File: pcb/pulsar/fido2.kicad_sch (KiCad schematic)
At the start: 16 parts, among them J1 FPC_10P_0.5mm, U1 ISO1540DR, U2 STM32L052K8T6, U3 ATECC608B-MAHDA-S

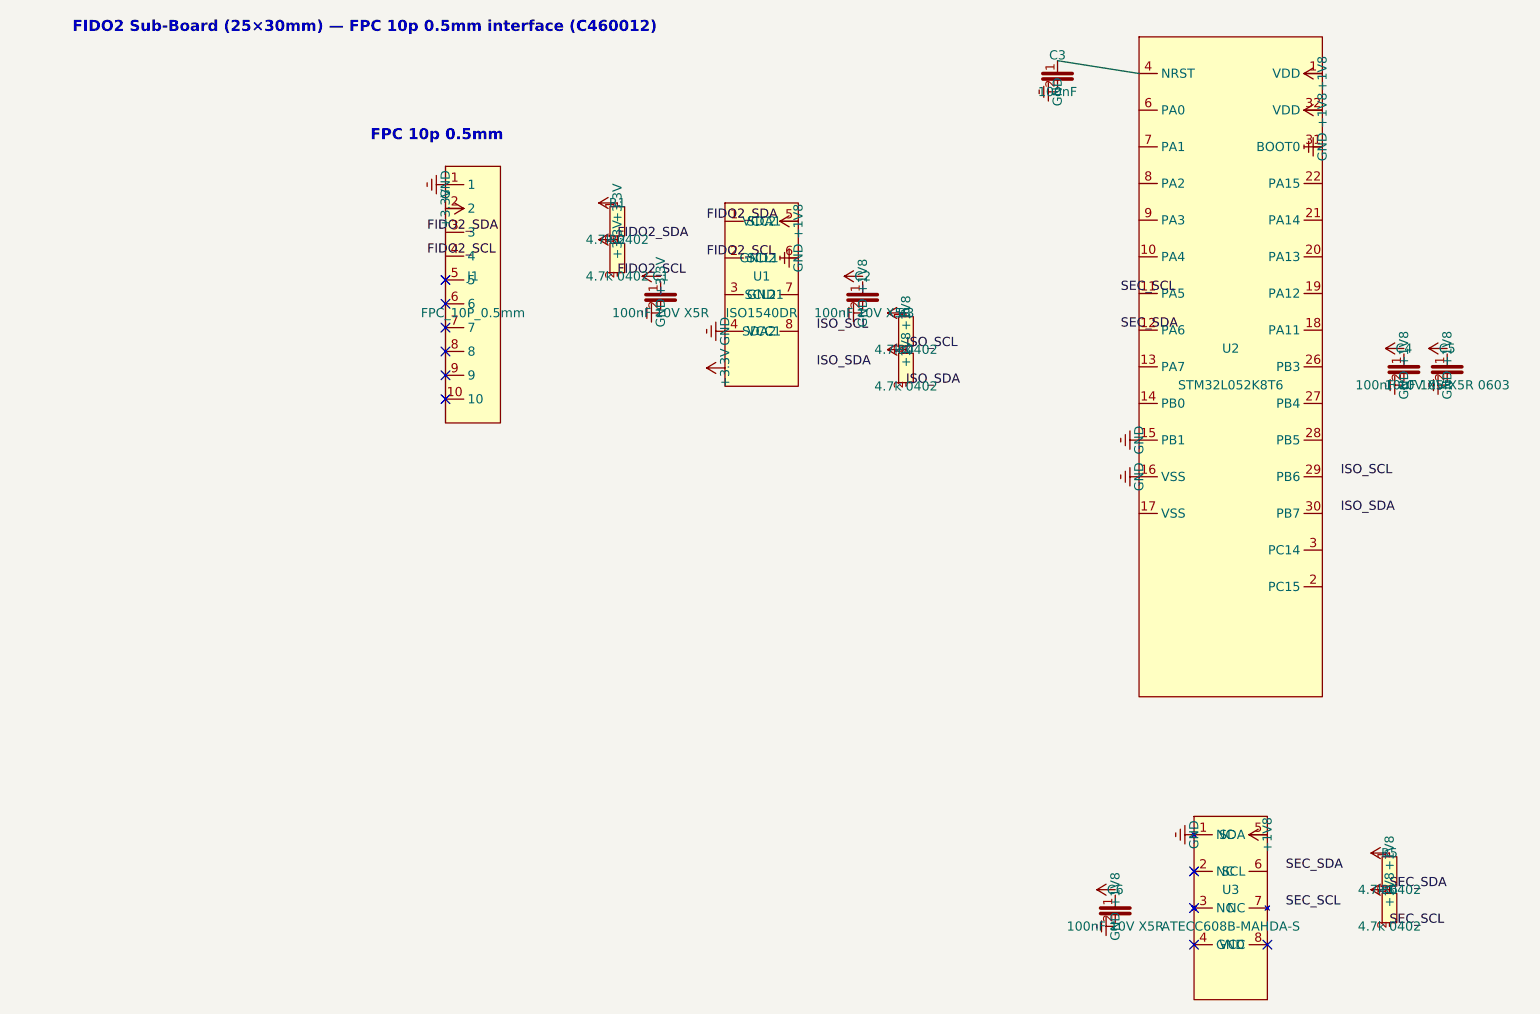
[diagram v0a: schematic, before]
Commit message: feat: let everything to route
Signed-off-by: Axel Ibarrondo <135344010+Axel84727@users.noreply.github.com>
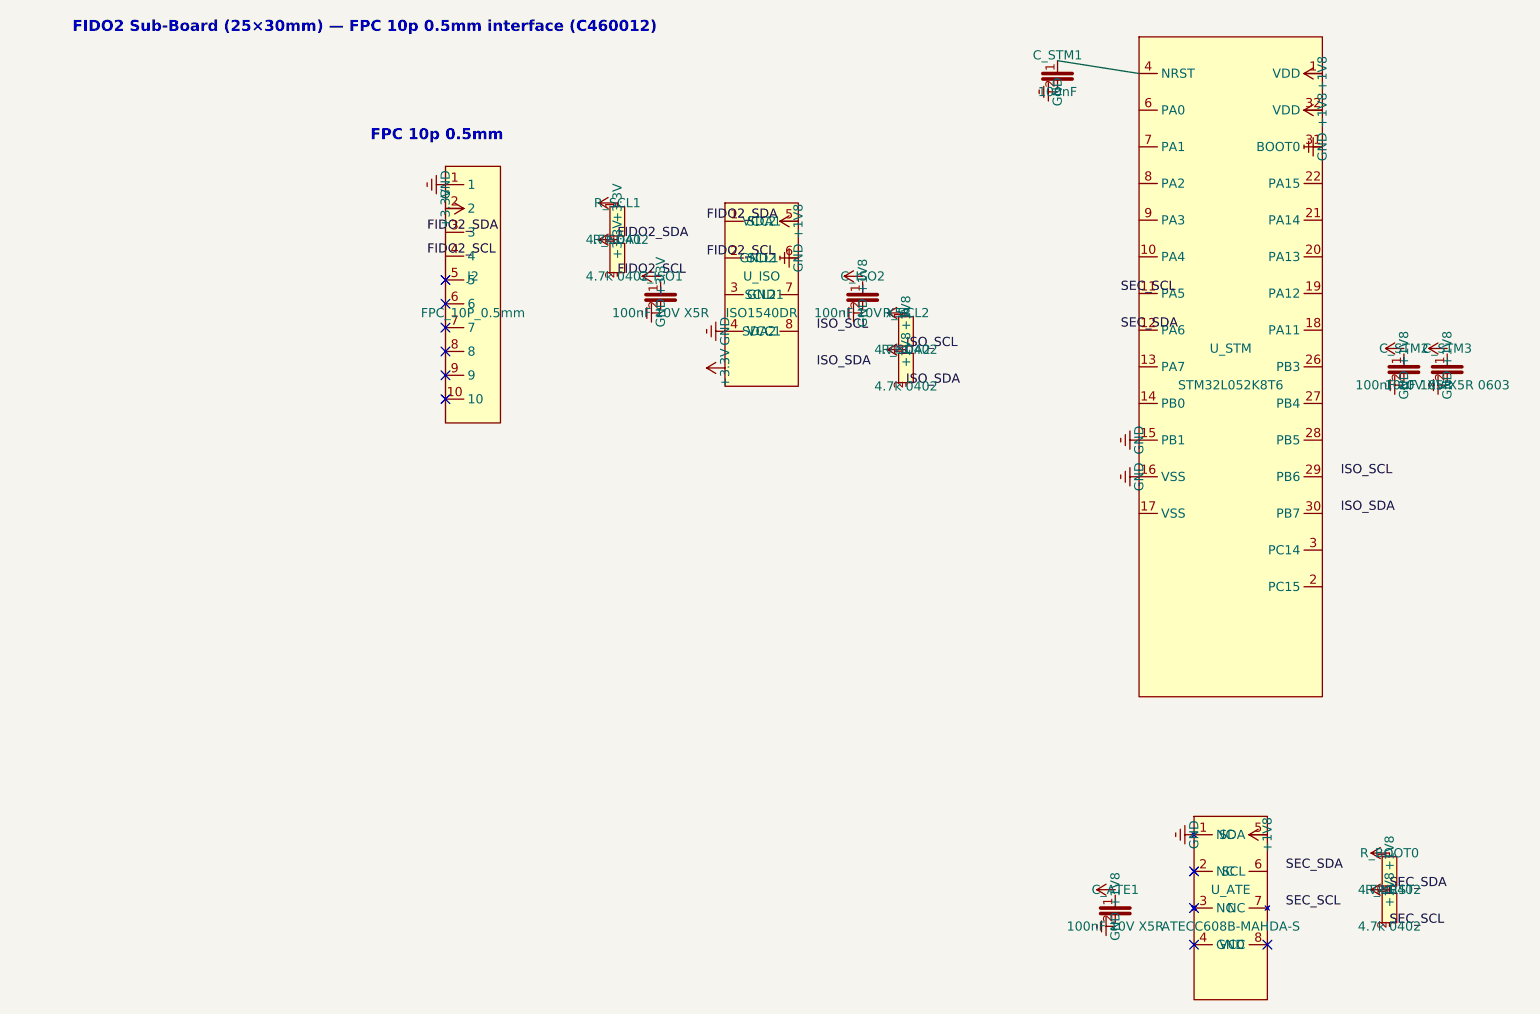
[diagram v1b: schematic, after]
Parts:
- renumbered C6 to C_ATE1, C1 to C_ISO1, C2 to C_ISO2, C3 to C_STM1, C4 to C_STM2, C5 to C_STM3, J1 to J2, R5 to R_BOOT0, R6 to R_NRST, R1 to R_SCL1, R3 to R_SCL2, R2 to R_SDA1, R4 to R_SDA2, U3 to U_ATE, U1 to U_ISO, U2 to U_STM
